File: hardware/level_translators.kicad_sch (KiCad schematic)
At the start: 30 parts, among them U10 UM3304, U11 UM3304, U12 UM3304, U13 UM3304, U14 UM3304, U15 UM3304

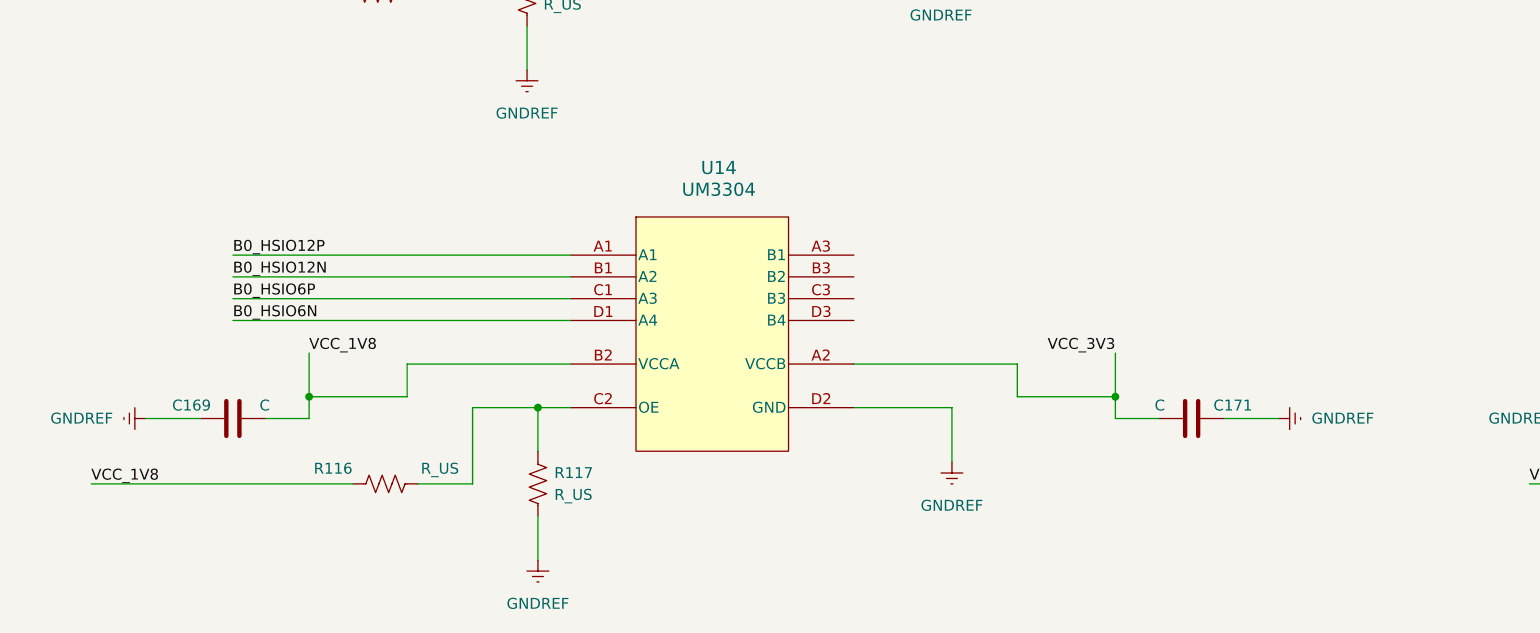
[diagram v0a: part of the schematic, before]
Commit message: need some I/O adjustments
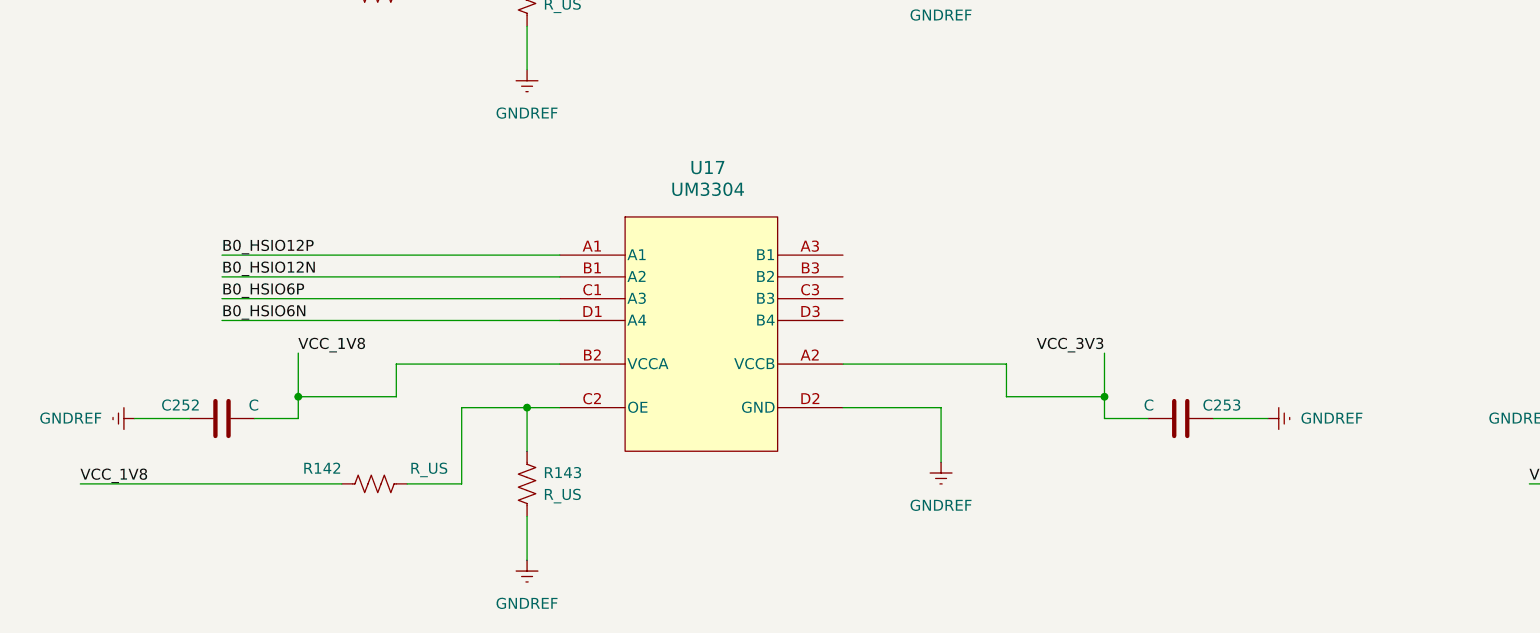
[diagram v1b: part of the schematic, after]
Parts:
- removed C169, C171: C, symbol Device:C
- removed R116, R117: R_US, symbol Device:R_US
- removed U14: UM3304, CSP12_1P9X1P4_USC, symbol payload-sym:UM3304
- added C252, C253: C, symbol Device:C
- added R142, R143: R_US, symbol Device:R_US
- added U17: UM3304, CSP12_1P9X1P4_USC, symbol payload-sym:UM3304
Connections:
- net B0_HSIO12N: now also U17.B1 (A2)
- net B0_HSIO12P: now also U17.A1
- net B0_HSIO6N: now also U17.D1 (A4)
- net B0_HSIO6P: now also U17.C1 (A3)
- net GNDREF: now also C252.2, C253.2, R143.1, U17.D2 (GND)
- net VCC_1V8: now also C252.1, R142.1, U17.B2 (VCCA)
- net VCC_3V3: now also C253.1, U17.A2 (VCCB)
- new net: R142.2, R143.2, U17.C2 (OE)
